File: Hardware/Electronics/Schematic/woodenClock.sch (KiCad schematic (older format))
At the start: 0 parts

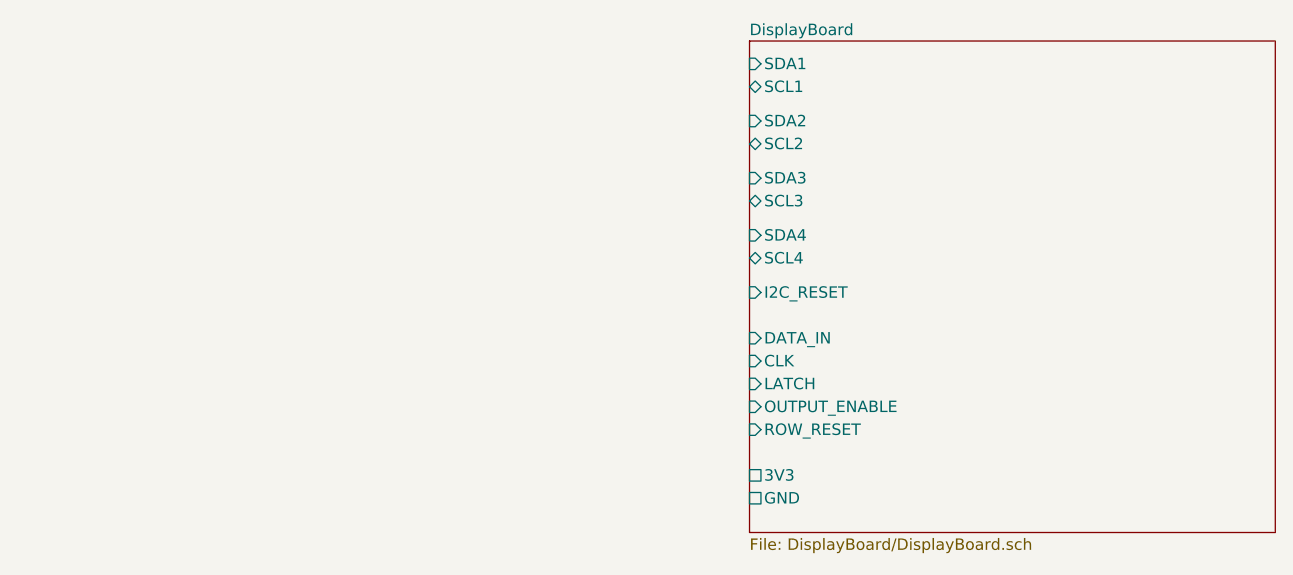
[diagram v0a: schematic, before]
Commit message: Schematic update -- start of the main board designe
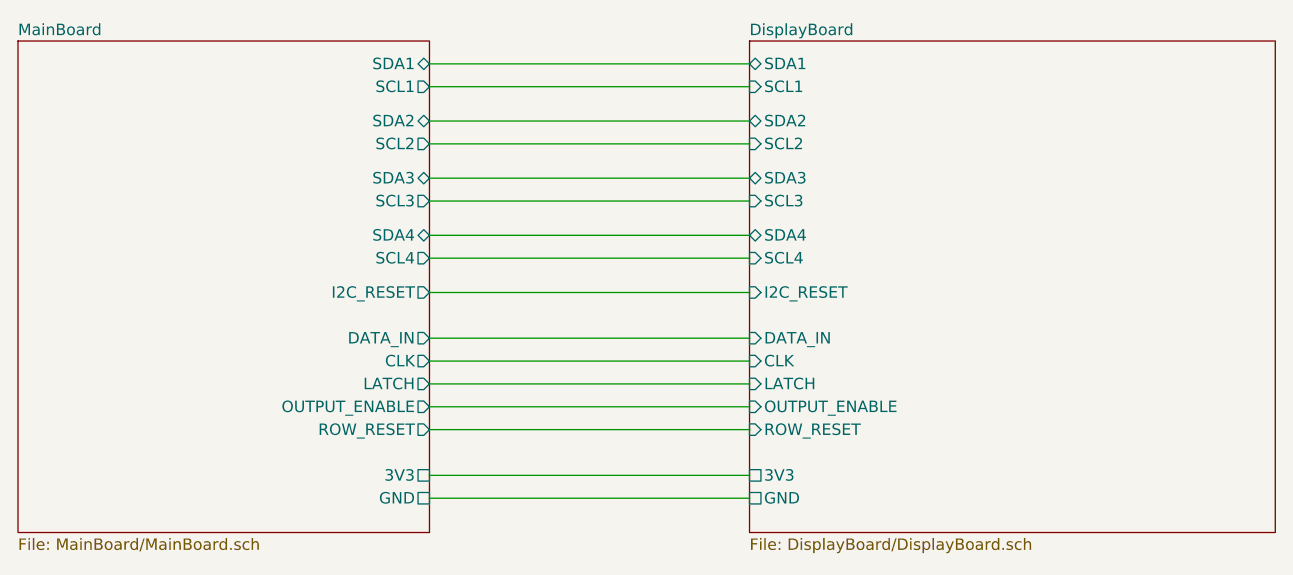
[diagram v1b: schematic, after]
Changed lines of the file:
@@
 EESchema Schematic File Version 4
-LIBS:main-cache
 EELAYER 26 0
 EELAYER END
 $Descr A4 11693 8268
 encoding utf-8
-Sheet 1 7
+Sheet 1 8
 Title "Wooden clock"
 Date "2018-10-21"
@@
 F0 "DisplayBoard" 50
 F1 "DisplayBoard/DisplayBoard.sch" 50
-F2 "SDA1" I L 8150 3000 50
-F3 "SCL1" B L 8150 3100 50
-F4 "SDA2" I L 8150 3250 50
-F5 "SDA3" I L 8150 3500 50
-F6 "SDA4" I L 8150 3750 50
+F2 "SDA1" B L 8150 3000 50
+F3 "SCL1" I L 8150 3100 50
+F4 "SDA2" B L 8150 3250 50
+F5 "SDA3" B L 8150 3500 50
+F6 "SDA4" B L 8150 3750 50
 F7 "OUTPUT_ENABLE" I L 8150 4500 50
 F8 "LATCH" I L 8150 4400 50
@@
 F13 "3V3" U L 8150 4800 50
 F14 "GND" U L 8150 4900 50
-F15 "SCL2" B L 8150 3350 50
-F16 "SCL3" B L 8150 3600 50
-F17 "SCL4" B L 8150 3850 50
+F15 "SCL2" I L 8150 3350 50
+F16 "SCL3" I L 8150 3600 50
+F17 "SCL4" I L 8150 3850 50
 $EndSheet
+$Sheet
+S 4950 2900 1800 2150
+U 5CCD8EC9
+F0 "MainBoard" 50
+F1 "MainBoard/MainBoard.sch" 50
+F2 "SDA1" B R 6750 3000 50
+F3 "SCL1" O R 6750 3100 50
+F4 "SDA2" B R 6750 3250 50
+F5 "SCL2" O R 6750 3350 50
+F6 "SDA3" B R 6750 3500 50
+F7 "SCL3" O R 6750 3600 50
+F8 "SDA4" B R 6750 3750 50
+F9 "SCL4" O R 6750 3850 50
+F10 "I2C_RESET" O R 6750 4000 50
+F11 "DATA_IN" O R 6750 4200 50
+F12 "CLK" O R 6750 4300 50
+F13 "LATCH" O R 6750 4400 50
+F14 "OUTPUT_ENABLE" O R 6750 4500 50
+F15 "ROW_RESET" O R 6750 4600 50
+F16 "3V3" U R 6750 4800 50
+F17 "GND" U R 6750 4900 50
+$EndSheet
+Wire Wire Line
+	6750 3000 8150 3000
+Wire Wire Line
+	8150 3100 6750 3100
+Wire Wire Line
+	6750 3250 8150 3250
+Wire Wire Line
+	8150 3350 6750 3350
+Wire Wire Line
+	6750 3500 8150 3500
+Wire Wire Line
+	8150 3600 6750 3600
+Wire Wire Line
+	6750 3750 8150 3750
+Wire Wire Line
+	8150 3850 6750 3850
+Wire Wire Line
+	6750 4000 8150 4000
+Wire Wire Line
+	6750 4200 8150 4200
+Wire Wire Line
+	6750 4300 8150 4300
+Wire Wire Line
+	6750 4400 8150 4400
+Wire Wire Line
+	6750 4500 8150 4500
+Wire Wire Line
+	6750 4600 8150 4600
+Wire Wire Line
+	6750 4800 8150 4800
+Wire Wire Line
+	6750 4900 8150 4900
 $EndSCHEMATC
